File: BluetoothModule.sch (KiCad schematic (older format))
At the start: 21 parts, among them J8 SW_DIP_x01, J9 SW_DIP_x01, U17 BM64SPKS1MCx, U5 APX803L

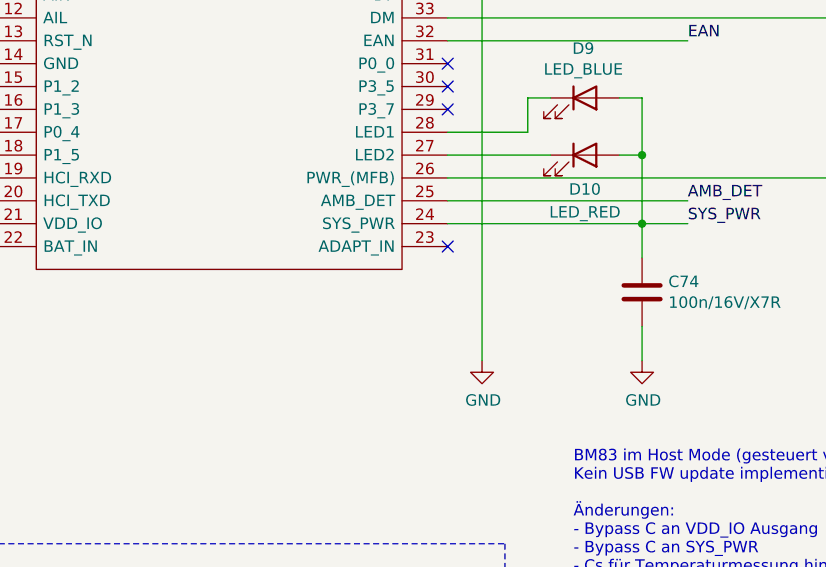
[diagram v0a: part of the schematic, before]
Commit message: [add:] annotations, corrections from testing
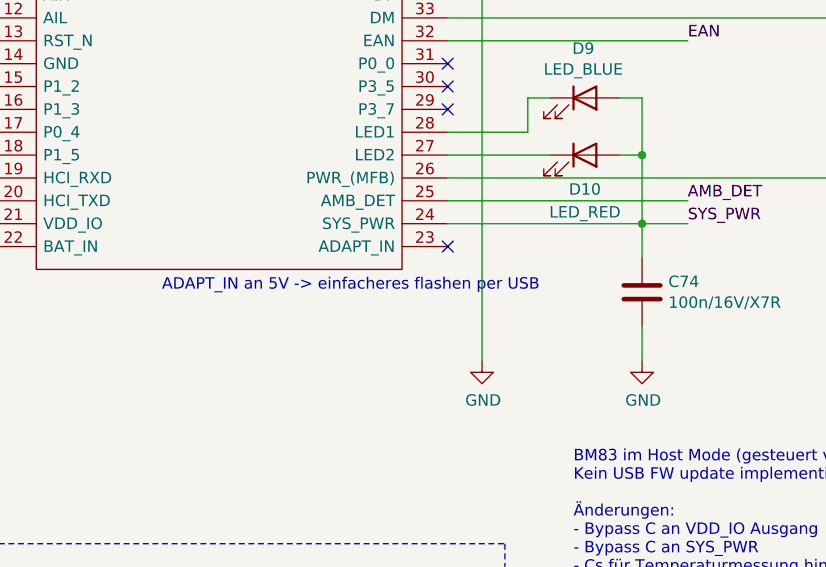
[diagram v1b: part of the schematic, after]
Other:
- note added: "ADAPT_IN an 5V -> einfacheres flashen per USB"
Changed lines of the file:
@@
 Data
 89 50 4E 47 0D 0A 1A 0A 00 00 00 0D 49 48 44 52 00 00 05 D7 00 00 02 9F 08 02 00 00 00 03 DC 66
-88 00 00 00 03 73 42 49 54 08 08 08 DB E1 4F E0 00 00 00 09 70 48 59 73 00 00 19 D6 00 00 19 D6
-01 18 D1 CA ED 00 00 20 00 49 44 41 54 78 9C EC 9D 79 B4 65 55 75 EE BF D5 ED E6 34 B7 A9 AA 5B
+88 00 00 00 03 73 42 49 54 08 08 08 DB E1 4F E0 00 00 00 09 70 48 59 73 00 00 19 C8 00 00 19 C8
+01 F5 4C 96 D9 00 00 20 00 49 44 41 54 78 9C EC 9D 79 B4 65 55 75 EE BF D5 ED E6 34 B7 A9 AA 5B
 45 53 20 28 3D F6 B4 F6 82 44 11 44 C4 D8 12 8D 31 B6 B1 4B 24 EA 88 26 1A 9B 3C 21 1A 62 8B 8A
 02 2A 18 14 45 44 11 95 C4 5E 04 D4 A0 B4 A2 02 45 41 59 50 54 DD 5B F7 DE D3 EC BD 57 37 E7 FB
@@
 EndData
 $EndBitmap
+Text Notes 4400 4150 0    50   ~ 0
+ADAPT_IN an 5V -> einfacheres flashen per USB
 $EndSCHEMATC
